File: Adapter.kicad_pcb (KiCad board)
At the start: 2 copper layers, 35.3 x 31.2 mm, 7 parts, among them J1 Conn_01x04, J2 Conn_01x06, J3 Conn_01x10, J4 Conn_01x10, J5 Conn_01x10, U1 NRF52832_E73-2G4M04S1B

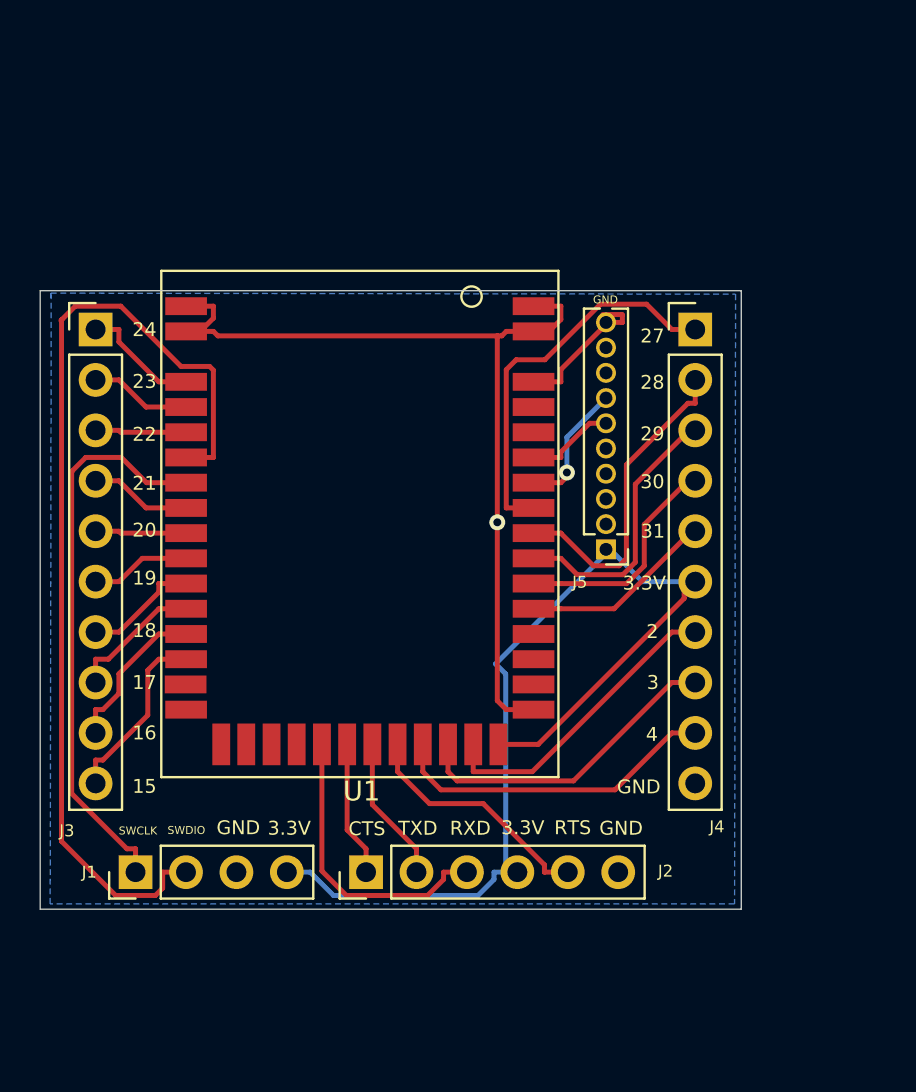
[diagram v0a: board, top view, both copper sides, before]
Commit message: Version 2.0 updated.
PCB design updated.
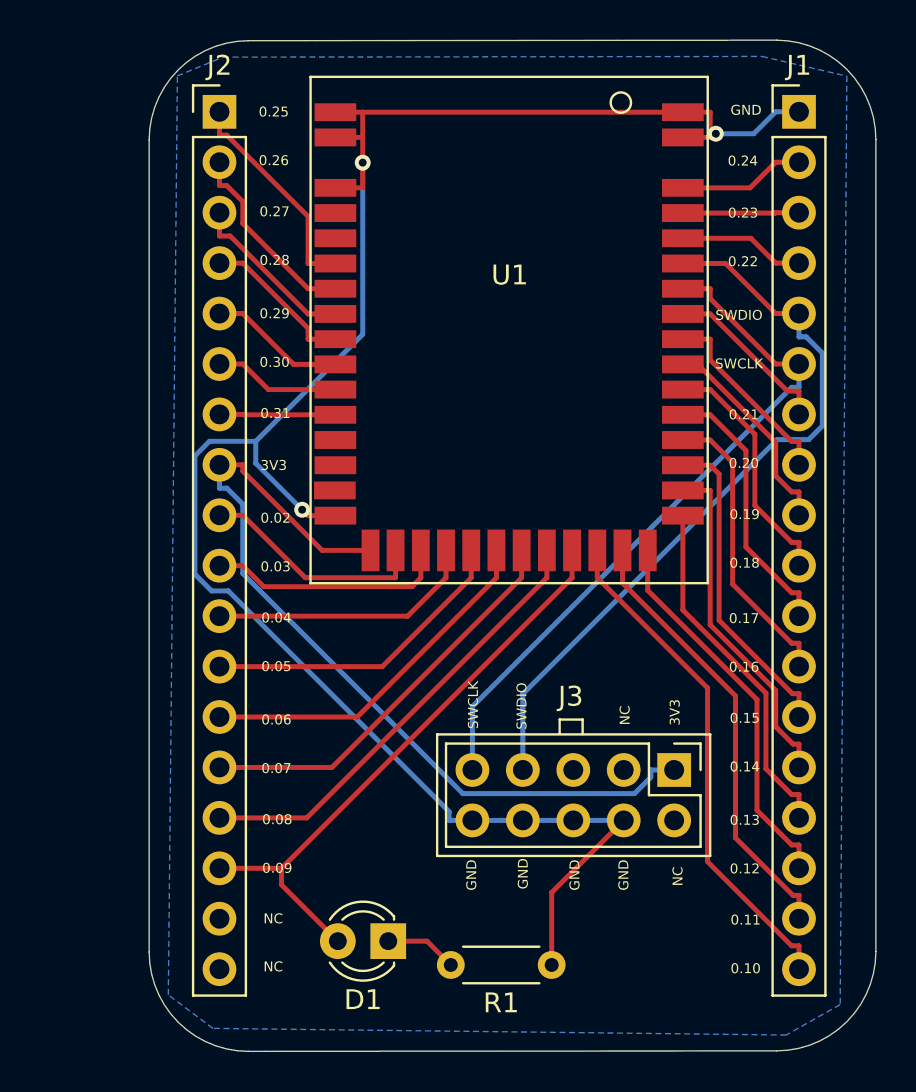
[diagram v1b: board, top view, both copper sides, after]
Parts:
- removed J4: Conn_01x10, Connector_PinHeader_2.54mm:PinHeader_1x10_P2.54mm_Vertical
- removed J5: Conn_01x10, Connector_PinHeader_1.27mm:PinHeader_1x10_P1.27mm_Vertical
- removed the REF** at (144.7, 92.2)
- added D1: LED, LED_THT:LED_D3.0mm, F.Cu at (145.9, 113.6)
- added R1: R, Resistor_THT:R_Axial_DIN0204_L3.6mm_D1.6mm_P5.08mm_Horizontal, F.Cu at (154.1, 114.8)
- added REF**: OSHW-Logo2_24.3x20mm_SilkScreen, Symbol:OSHW-Logo2_24.3x20mm_SilkScreen, B.Cu at (152.7, 79.5)
- added REF**: KiCad-Logo2_5mm_SilkScreen, Symbol:KiCad-Logo2_5mm_SilkScreen, B.Cu at (153.2, 92.0)
- J1: value Conn_01x04 -> Conn_01x18; footprint Connector_PinHeader_2.54mm:PinHeader_1x04_P2.54mm_Vertical -> Connector_PinHeader_2.54mm:PinHeader_1x18_P2.54mm_Vertical
- J2: value Conn_01x06 -> Conn_01x18; footprint Connector_PinHeader_2.54mm:PinHeader_1x06_P2.54mm_Vertical -> Connector_PinHeader_2.54mm:PinHeader_1x18_P2.54mm_Vertical
- J3: value Conn_01x10 -> Conn_02x05_Odd_Even; footprint Connector_PinHeader_2.54mm:PinHeader_1x10_P2.54mm_Vertical -> Connector_PinHeader_2.54mm:PinHeader_2x05_P2.54mm_Vertical
- moved J1 50.8 mm to (166.5, 71.8), turned to 0 degrees
- moved J2 39.0 mm to (137.4, 71.8), turned to 0 degrees
- moved J3 36.6 mm to (160.3, 104.9), turned to 270 degrees
- moved U1 12.3 mm to (151.9, 79.5)
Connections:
- J1 pad 1: /SWDCLK -> GND
- J1 pad 2: /SWDIO -> /42
- J1 pad 3: GND -> /41
- J1 pad 4: /+3.3VCC -> /40
- J2 pad 1: /7_CTS -> /6
- J2 pad 2: /6_TX -> /7
- J2 pad 3: /8_RX -> /8
- J2 pad 4: /+3.3VCC -> /9
- J2 pad 5: /5_RTS -> /10
- J2 pad 6: GND -> /11
- J3 pad 1: /24 -> /+3.3VCC
- J3 pad 10: /15 -> GND
- J3 pad 2: /23 -> Net-(J3-Pad2)
- J3 pad 3: /22 -> Net-(J3-Pad3)
- J3 pad 4: /21 -> GND
- J3 pad 5: /20 -> Net-(J3-Pad5)
- J3 pad 6: /19 -> GND
- J3 pad 7: /18 -> /39
- J3 pad 8: /17 -> GND
- J3 pad 9: /16 -> /38
- U1 pad 10: /29 -> /10
- U1 pad 11: /30 -> /11
- U1 pad 12: /31 -> /12
- U1 pad 18: /2 -> /18
- U1 pad 19: /3 -> /19
- U1 pad 20: /4 -> /20
- U1 pad 21: /5_RTS -> /21
- U1 pad 22: /6_TX -> /22
- U1 pad 23: /7_CTS -> /23
- U1 pad 24: /8_RX -> /24
- U1 pad 25: Net-(U1-Pad25) -> /25
- U1 pad 26: Net-(U1-Pad26) -> /26
- U1 pad 27: /11 -> /27
- U1 pad 28: /12 -> /28
- U1 pad 29: /13 -> /29
- U1 pad 30: /14 -> /30
- U1 pad 31: /15 -> /31
- U1 pad 32: /16 -> /32
- U1 pad 33: /17 -> /33
- U1 pad 34: /18 -> /34
- U1 pad 35: /19 -> /35
- U1 pad 36: /20 -> /36
- U1 pad 37: /21 -> /37
- U1 pad 38: /SWDCLK -> /38
- U1 pad 39: /SWDIO -> /39
- U1 pad 40: /22 -> /40
- U1 pad 41: /23 -> /41
- U1 pad 42: /24 -> /42
- U1 pad 6: /25 -> /6
- U1 pad 7: /26 -> /7
- U1 pad 8: /27 -> /8
- U1 pad 9: /28 -> /9
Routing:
- net /SWDIO: track 49.7 -> 0.00 mm
- net GND: track 53.1 -> 100.6 mm, vias 1 -> 3
- net /39: track 0.00 -> 37.8 mm
- net /38: track 0.00 -> 35.2 mm
- net /SWDCLK: track 28.4 -> 0.00 mm
- net /25: track 4.52 -> 30.0 mm
- net /26: track 6.58 -> 25.5 mm, vias 1 -> 0
- net /24: track 6.02 -> 22.9 mm
- net /4: track 16.7 -> 0.00 mm
- net /3: track 16.1 -> 0.00 mm
- net /2: track 15.5 -> 0.00 mm
- net /23: track 5.12 -> 20.6 mm
- net /8_RX: track 14.9 -> 0.00 mm
- net /32: track 0.00 -> 14.9 mm
- net /22: track 4.60 -> 18.2 mm
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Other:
- board size 35.3 x 31.2 mm -> 36.6 x 50.9 mm
- board text added: "0.02"
- board text added: "0.03"
- board text added: "0.04"
- board text added: "0.05"
- board text added: "0.06"
- board text added: "0.07"
- board text added: "0.08"
- board text added: "0.09"
- board text added: "0.10"
- board text added: "0.11"
- board text added: "0.12"
- board text added: "0.13"
- board text added: "0.14"
- board text added: "0.15"
- board text added: "0.16"
- board text added: "0.17"
- board text added: "0.18"
- board text added: "0.19"
- board text added: "0.20"
- board text added: "0.21"
- board text added: "0.22"
- board text added: "0.23"
- board text added: "0.24"
- board text added: "0.25"
- board text added: "0.26"
- board text added: "0.27"
- board text added: "0.28"
- board text added: "0.29"
- board text added: "0.30"
- board text added: "0.31"
- board text added: "3V3"
- board text added: "NC"
- board text added: "NRF Adapter"
- board text added: "Revision 2"
- board text removed: "15"
- board text removed: "16"
- board text removed: "17"
- board text removed: "18"
- board text removed: "19"
- board text removed: "2"
- board text removed: "20"
- board text removed: "21"
- board text removed: "22"
- board text removed: "23"
- board text removed: "24"
- board text removed: "27"
- board text removed: "28"
- board text removed: "29"
- board text removed: "3"
- board text removed: "3.3V"
- board text removed: "30"
- board text removed: "31"
- board text removed: "4"
- board text removed: "CTS"
- board text removed: "NRF Adapter Rev 1.0"
- board text removed: "RTS"
- board text removed: "RXD"
- board text removed: "TXD"
